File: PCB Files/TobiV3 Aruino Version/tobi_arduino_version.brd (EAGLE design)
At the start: 103 x 74 mm, 45 parts

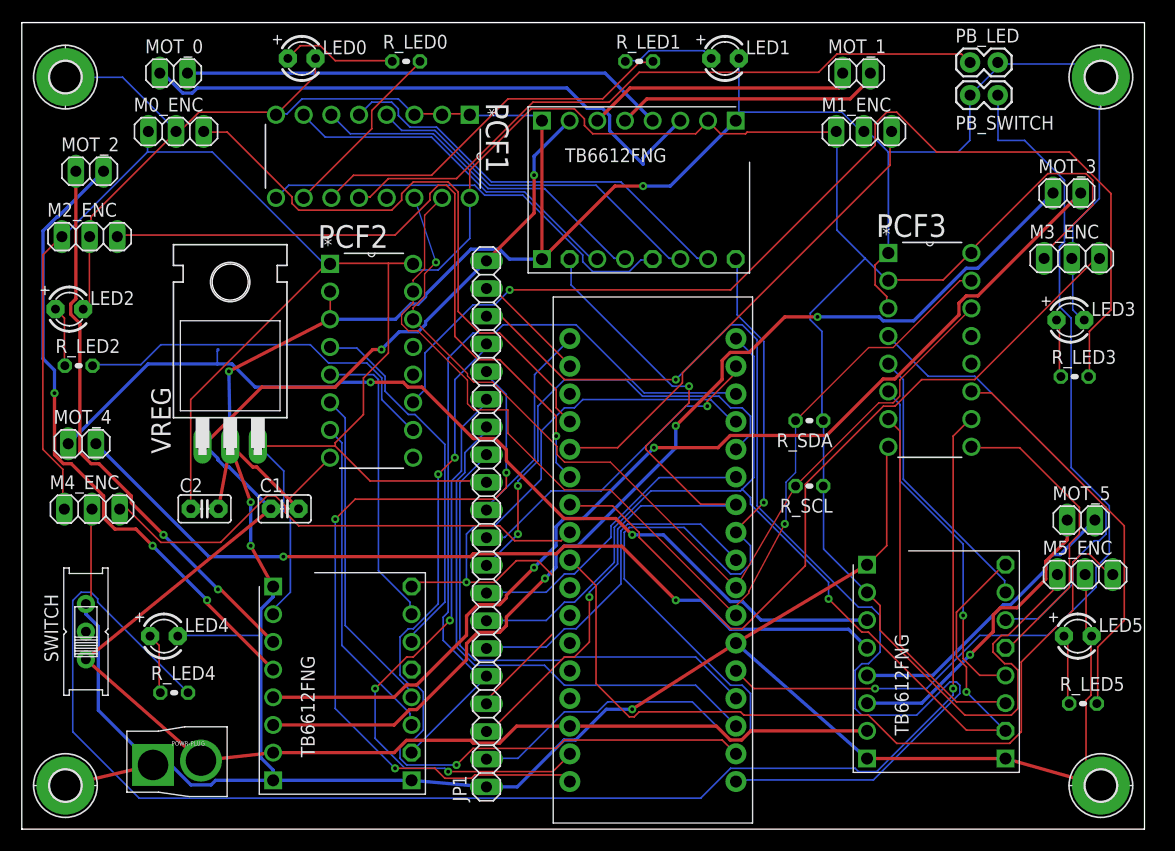
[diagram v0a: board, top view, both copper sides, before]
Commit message: rip up main board and try again...
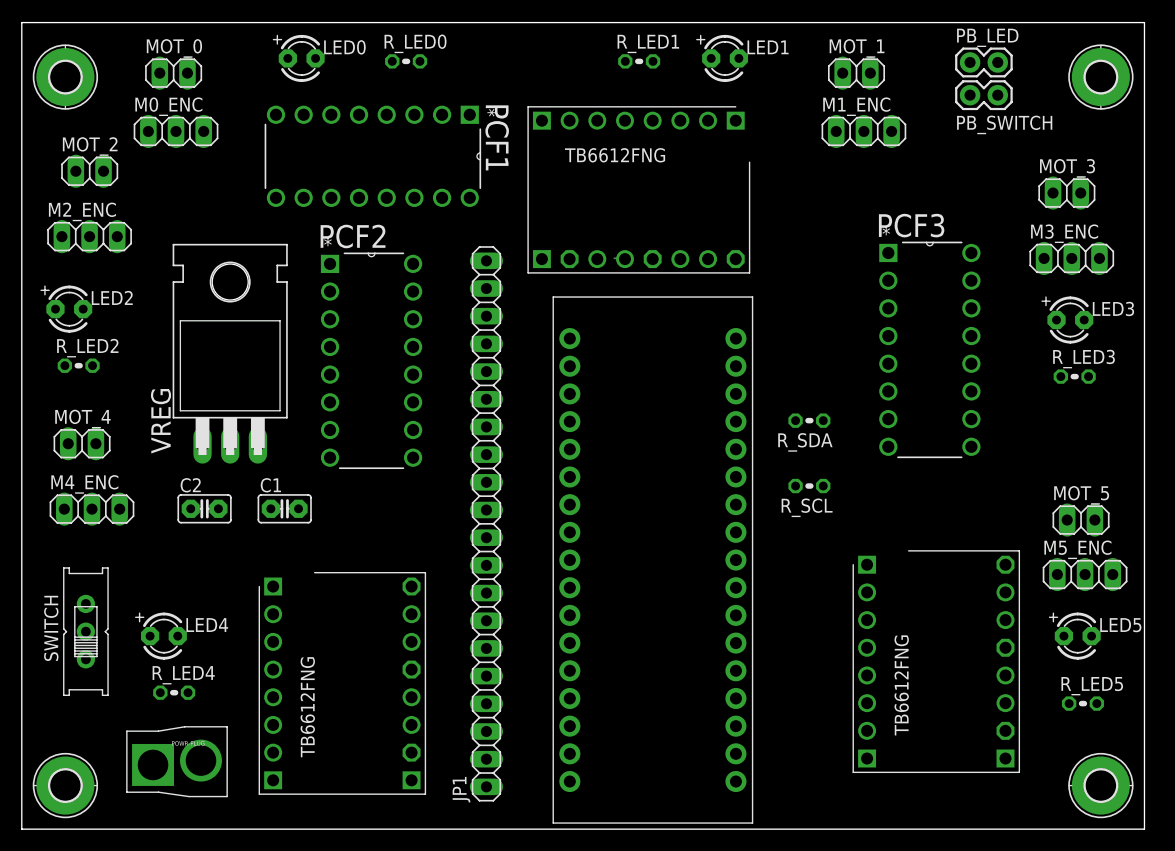
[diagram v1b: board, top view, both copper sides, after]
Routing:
- net GND: track 478.9 -> 0.00 mm, vias 5 -> 0
- net VCC: track 325.6 -> 0.09 mm
- net V_MOT: track 159.4 -> 0.38 mm, vias 2 -> 0
- net LED4: track 140.5 -> 0.00 mm, vias 1 -> 0
- net MOSI: track 106.3 -> 0.00 mm, vias 1 -> 0
- net LED3: track 99.0 -> 0.00 mm, vias 1 -> 0
- net M5_PWM: track 99.0 -> 0.00 mm, vias 2 -> 0
- net SDA: track 98.4 -> 0.00 mm, vias 1 -> 0
- net M0_PWM: track 96.4 -> 0.00 mm, vias 1 -> 0
- net M3_A: track 96.3 -> 0.00 mm, vias 3 -> 0
- net M3_B: track 96.1 -> 0.00 mm, vias 2 -> 0
- net RESET: track 89.3 -> 0.00 mm, vias 1 -> 0
- net M4_A: track 88.3 -> 0.00 mm, vias 2 -> 0
- net SCL: track 87.3 -> 0.00 mm, vias 1 -> 0
- net M4_B: track 79.3 -> 0.00 mm, vias 2 -> 0
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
